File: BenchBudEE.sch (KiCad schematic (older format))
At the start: 0 parts

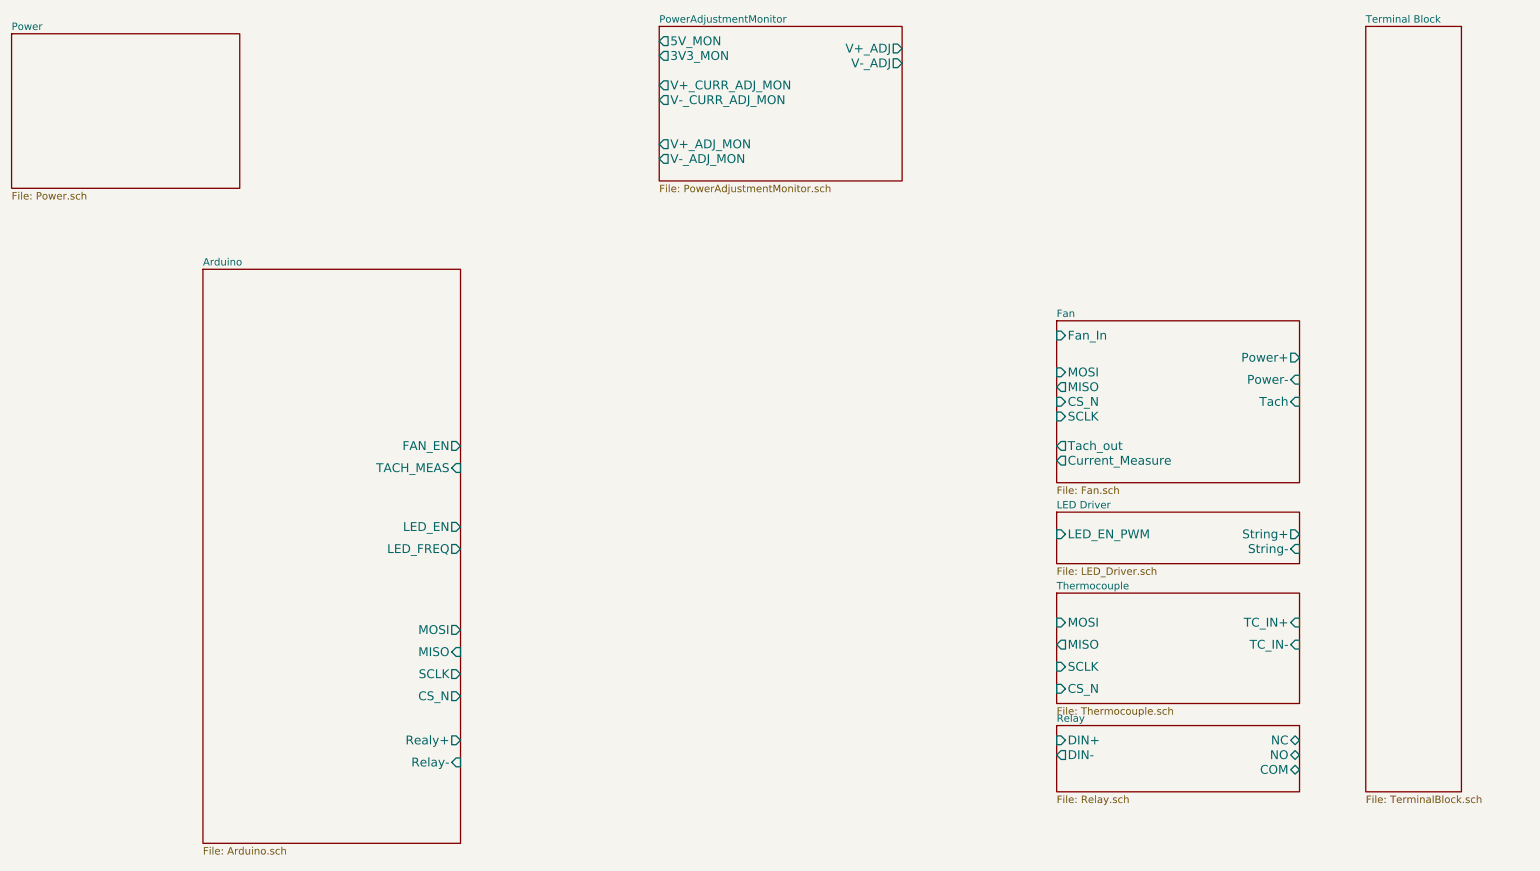
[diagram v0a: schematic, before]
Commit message: Module 3, Unit 9: Understanding The Arduino Module
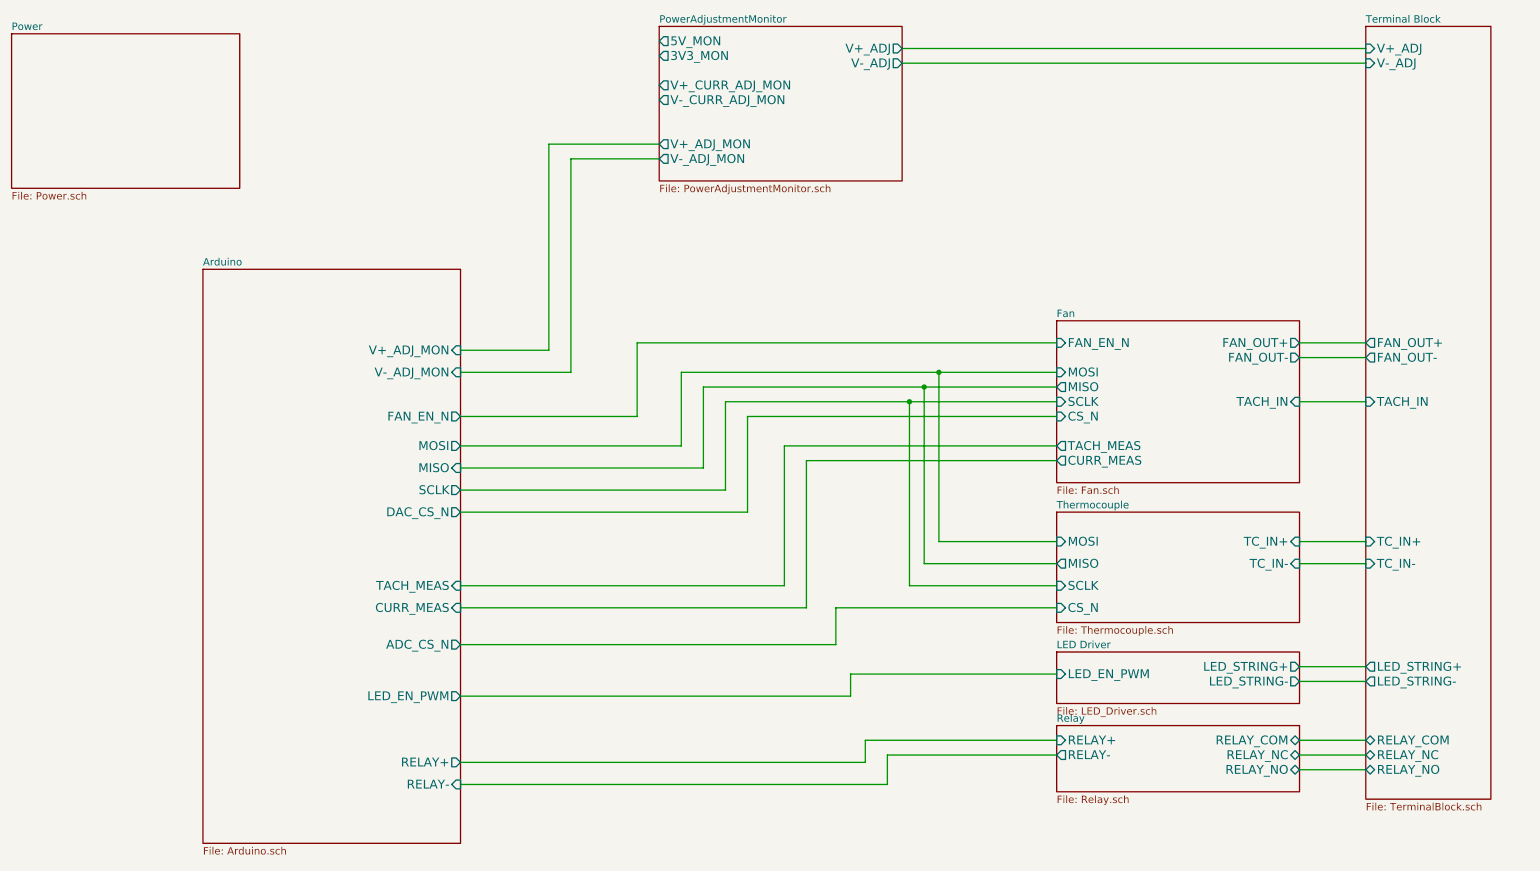
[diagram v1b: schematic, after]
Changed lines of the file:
@@
 $EndDescr
 $Sheet
-S 2100 2700 1750 3900
-U 52FFA904
-F0 "Arduino" 50
-F1 "Arduino.sch" 50
-F2 "Realy+" O R 3850 5900 60
-F3 "Relay-" I R 3850 6050 60
-F4 "MOSI" O R 3850 5150 60
-F5 "MISO" I R 3850 5300 60
-F6 "SCLK" O R 3850 5450 60
-F7 "CS_N" O R 3850 5600 60
-F8 "LED_EN" O R 3850 4450 60
-F9 "LED_FREQ" O R 3850 4600 60
-F10 "FAN_EN" O R 3850 3900 60
-F11 "TACH_MEAS" I R 3850 4050 60
-$EndSheet
-$Sheet
-S 7900 4900 1650 750
+S 7900 4350 1650 750
 U 52FFA9C4
 F0 "Thermocouple" 50
 F1 "Thermocouple.sch" 50
-F2 "TC_IN+" I R 9550 5100 60
-F3 "TC_IN-" I R 9550 5250 60
-F4 "MOSI" I L 7900 5100 60
-F5 "MISO" O L 7900 5250 60
-F6 "SCLK" I L 7900 5400 60
-F7 "CS_N" I L 7900 5550 60
+F2 "TC_IN+" I R 9550 4550 60
+F3 "TC_IN-" I R 9550 4700 60
+F4 "MOSI" I L 7900 4550 60
+F5 "MISO" O L 7900 4700 60
+F6 "SCLK" I L 7900 4850 60
+F7 "CS_N" I L 7900 5000 60
 $EndSheet
 $Sheet
@@
 F0 "Relay" 50
 F1 "Relay.sch" 50
-F2 "DIN+" I L 7900 5900 60
-F3 "DIN-" O L 7900 6000 60
-F4 "NC" B R 9550 5900 60
-F5 "NO" B R 9550 6000 60
-F6 "COM" B R 9550 6100 60
+F2 "RELAY_NC" B R 9550 6000 60
+F3 "RELAY_NO" B R 9550 6100 60
+F4 "RELAY_COM" B R 9550 5900 60
+F5 "RELAY+" I L 7900 5900 60
+F6 "RELAY-" O L 7900 6000 60
 $EndSheet
 $Sheet
@@
 $EndSheet
 $Sheet
-S 10000 1050 650  5200
+S 10000 1050 850  5250
 U 52FFAB03
 F0 "Terminal Block" 50
 F1 "TerminalBlock.sch" 50
-$EndSheet
-$Sheet
-S 7900 4350 1650 350
+F2 "V+_ADJ" I L 10000 1200 60
+F3 "V-_ADJ" I L 10000 1300 60
+F4 "FAN_OUT+" O L 10000 3200 60
+F5 "FAN_OUT-" O L 10000 3300 60
+F6 "TACH_IN" I L 10000 3600 60
+F7 "LED_STRING+" O L 10000 5400 60
+F8 "LED_STRING-" O L 10000 5500 60
+F9 "TC_IN+" I L 10000 4550 60
+F10 "TC_IN-" I L 10000 4700 60
+F11 "RELAY_COM" B L 10000 5900 60
+F12 "RELAY_NO" B L 10000 6100 60
+F13 "RELAY_NC" B L 10000 6000 60
+$EndSheet
+$Sheet
+S 7900 5300 1650 350
 U 52FFAA9A
 F0 "LED Driver" 50
 F1 "LED_Driver.sch" 50
-F2 "String+" O R 9550 4500 60
-F3 "String-" I R 9550 4600 60
-F4 "LED_EN_PWM" I L 7900 4500 60
+F2 "LED_EN_PWM" I L 7900 5450 60
+F3 "LED_STRING+" O R 9550 5400 60
+F4 "LED_STRING-" O R 9550 5500 60
 $EndSheet
 $Sheet
@@
 F0 "Fan" 50
 F1 "Fan.sch" 50
-F2 "Power+" O R 9550 3300 60
-F3 "Power-" I R 9550 3450 60
-F4 "Tach" I R 9550 3600 60
-F5 "Tach_out" O L 7900 3900 60
-F6 "Fan_In" I L 7900 3150 60
-F7 "Current_Measure" O L 7900 4000 60
-F8 "MOSI" I L 7900 3400 60
-F9 "MISO" O L 7900 3500 60
-F10 "CS_N" I L 7900 3600 60
-F11 "SCLK" I L 7900 3700 60
+F2 "MOSI" I L 7900 3400 60
+F3 "MISO" O L 7900 3500 60
+F4 "CS_N" I L 7900 3700 60
+F5 "SCLK" I L 7900 3600 60
+F6 "FAN_OUT+" O R 9550 3200 60
+F7 "TACH_IN" I R 9550 3600 60
+F8 "TACH_MEAS" O L 7900 3900 60
+F9 "FAN_EN_N" I L 7900 3200 60
+F10 "CURR_MEAS" O L 7900 4000 60
+F11 "FAN_OUT-" O R 9550 3300 60
 $EndSheet
 $Sheet
@@
 F9 "V-_CURR_ADJ_MON" O L 5200 1550 60
 $EndSheet
+Wire Wire Line
+	6850 1200 10000 1200
+Wire Wire Line
+	6850 1300 10000 1300
+Wire Wire Line
+	9550 3200 10000 3200
+Wire Wire Line
+	9550 3300 10000 3300
+Wire Wire Line
+	9550 3600 10000 3600
+Wire Wire Line
+	9550 5900 10000 5900
+Wire Wire Line
+	9550 6000 10000 6000
+Wire Wire Line
+	9550 6100 10000 6100
+Wire Wire Line
+	3850 3250 4450 3250
+Wire Wire Line
+	4450 3250 4450 1850
+Wire Wire Line
+	4450 1850 5200 1850
+Wire Wire Line
+	5200 1950 4600 1950
+Wire Wire Line
+	4600 1950 4600 3400
+Wire Wire Line
+	4600 3400 3850 3400
+Wire Wire Line
+	3850 3700 5050 3700
+Wire Wire Line
+	5050 3700 5050 3200
+Wire Wire Line
+	5050 3200 7900 3200
+Wire Wire Line
+	3850 3900 5350 3900
+Wire Wire Line
+	5350 3900 5350 3400
+Wire Wire Line
+	5350 3400 7900 3400
+Wire Wire Line
+	3850 4050 5500 4050
+Wire Wire Line
+	5500 4050 5500 3500
+Wire Wire Line
+	5500 3500 7900 3500
+Wire Wire Line
+	3850 4200 5650 4200
+Wire Wire Line
+	5650 4200 5650 3600
+Wire Wire Line
+	5650 3600 7900 3600
+Wire Wire Line
+	3850 4350 5800 4350
+Wire Wire Line
+	5800 4350 5800 3700
+Wire Wire Line
+	5800 3700 7900 3700
+Wire Wire Line
+	9550 4550 10000 4550
+Wire Wire Line
+	10000 4700 9550 4700
+Wire Wire Line
+	9550 5400 10000 5400
+Wire Wire Line
+	9550 5500 10000 5500
+Wire Wire Line
+	7900 3900 6050 3900
+Wire Wire Line
+	6050 3900 6050 4850
+Wire Wire Line
+	6050 4850 3850 4850
+Wire Wire Line
+	7900 4000 6200 4000
+Wire Wire Line
+	6200 4000 6200 5000
+Wire Wire Line
+	6200 5000 3850 5000
+Wire Wire Line
+	7900 4550 7100 4550
+Wire Wire Line
+	7100 4550 7100 3400
+Connection ~ 7100 3400
+Wire Wire Line
+	7900 4700 7000 4700
+Wire Wire Line
+	7000 4700 7000 3500
+Connection ~ 7000 3500
+Wire Wire Line
+	7900 4850 6900 4850
+Wire Wire Line
+	6900 4850 6900 3600
+Connection ~ 6900 3600
+$Sheet
+S 2100 2700 1750 3900
+U 52FFA904
+F0 "Arduino" 50
+F1 "Arduino.sch" 50
+F2 "MOSI" O R 3850 3900 60
+F3 "MISO" I R 3850 4050 60
+F4 "SCLK" O R 3850 4200 60
+F5 "TACH_MEAS" I R 3850 4850 60
+F6 "RELAY+" O R 3850 6050 60
+F7 "RELAY-" I R 3850 6200 60
+F8 "FAN_EN_N" O R 3850 3700 60
+F9 "CURR_MEAS" I R 3850 5000 60
+F10 "V+_ADJ_MON" I R 3850 3250 60
+F11 "V-_ADJ_MON" I R 3850 3400 60
+F12 "LED_EN_PWM" O R 3850 5600 60
+F13 "DAC_CS_N" O R 3850 4350 60
+F14 "ADC_CS_N" O R 3850 5250 60
+$EndSheet
+Wire Wire Line
+	7900 5000 6400 5000
+Wire Wire Line
+	6400 5000 6400 5250
+Wire Wire Line
+	6400 5250 3850 5250
+Wire Wire Line
+	7900 5450 6500 5450
+Wire Wire Line
+	6500 5450 6500 5600
+Wire Wire Line
+	6500 5600 3850 5600
+Wire Wire Line
+	7900 5900 6600 5900
+Wire Wire Line
+	6600 5900 6600 6050
+Wire Wire Line
+	6600 6050 3850 6050
+Wire Wire Line
+	7900 6000 6750 6000
+Wire Wire Line
+	6750 6000 6750 6200
+Wire Wire Line
+	6750 6200 3850 6200
 $EndSCHEMATC
